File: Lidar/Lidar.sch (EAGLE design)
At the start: 4 parts

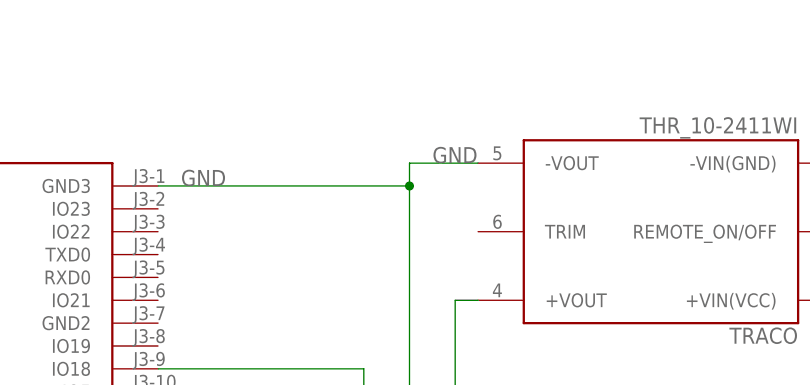
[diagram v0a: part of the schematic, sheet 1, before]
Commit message: board schematic
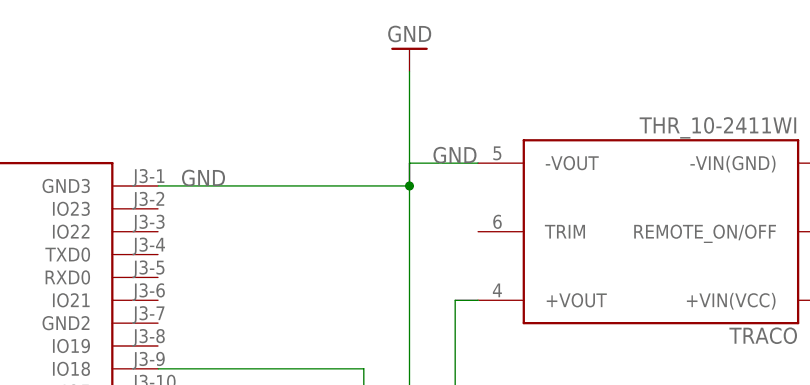
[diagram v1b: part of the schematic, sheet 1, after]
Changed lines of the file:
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@@
 <grid distance="0.1" unitdist="inch" unit="inch" style="lines" multiple="1" display="no" altdistance="0.01" altunitdist="inch" altunit="inch"/>
 <layers>
-<layer number="1" name="Top" color="4" fill="1" visible="yes" active="no"/>
-<layer number="16" name="Bottom" color="1" fill="1" visible="yes" active="no"/>
-<layer number="17" name="Pads" color="2" fill="1" visible="yes" active="no"/>
-<layer number="18" name="Vias" color="2" fill="1" visible="yes" active="no"/>
-<layer number="19" name="Unrouted" color="6" fill="1" visible="yes" active="no"/>
-<layer number="20" name="Dimension" color="15" fill="1" visible="yes" active="no"/>
-<layer number="21" name="tPlace" color="7" fill="1" visible="yes" active="no"/>
-<layer number="22" name="bPlace" color="7" fill="1" visible="yes" active="no"/>
-<layer number="23" name="tOrigins" color="15" fill="1" visible="yes" active="no"/>
-<layer number="24" name="bOrigins" color="15" fill="1" visible="yes" active="no"/>
-<layer number="25" name="tNames" color="7" fill="1" visible="yes" active="no"/>
-<layer number="26" name="bNames" color="7" fill="1" visible="yes" active="no"/>
-<layer number="27" name="tValues" color="7" fill="1" visible="yes" active="no"/>
-<layer number="28" name="bValues" color="7" fill="1" visible="yes" active="no"/>
+<layer number="1" name="Top" color="4" fill="1" visible="no" active="no"/>
+<layer number="16" name="Bottom" color="1" fill="1" visible="no" active="no"/>
+<layer number="17" name="Pads" color="2" fill="1" visible="no" active="no"/>
+<layer number="18" name="Vias" color="2" fill="1" visible="no" active="no"/>
+<layer number="19" name="Unrouted" color="6" fill="1" visible="no" active="no"/>
+<layer number="20" name="Dimension" color="15" fill="1" visible="no" active="no"/>
+<layer number="21" name="tPlace" color="7" fill="1" visible="no" active="no"/>
+<layer number="22" name="bPlace" color="7" fill="1" visible="no" active="no"/>
+<layer number="23" name="tOrigins" color="15" fill="1" visible="no" active="no"/>
+<layer number="24" name="bOrigins" color="15" fill="1" visible="no" active="no"/>
+<layer number="25" name="tNames" color="7" fill="1" visible="no" active="no"/>
+<layer number="26" name="bNames" color="7" fill="1" visible="no" active="no"/>
+<layer number="27" name="tValues" color="7" fill="1" visible="no" active="no"/>
+<layer number="28" name="bValues" color="7" fill="1" visible="no" active="no"/>
 <layer number="29" name="tStop" color="7" fill="3" visible="no" active="no"/>
 <layer number="30" name="bStop" color="7" fill="6" visible="no" active="no"/>
@@
 <layer number="35" name="tGlue" color="7" fill="4" visible="no" active="no"/>
 <layer number="36" name="bGlue" color="7" fill="5" visible="no" active="no"/>
-<layer number="37" name="tTest" color="7" fill="1" visible="yes" active="no"/>
-<layer number="38" name="bTest" color="7" fill="1" visible="yes" active="no"/>
+<layer number="37" name="tTest" color="7" fill="1" visible="no" active="no"/>
+<layer number="38" name="bTest" color="7" fill="1" visible="no" active="no"/>
 <layer number="39" name="tKeepout" color="4" fill="11" visible="no" active="no"/>
 <layer number="40" name="bKeepout" color="1" fill="11" visible="no" active="no"/>
@@
 <layer number="44" name="Drills" color="7" fill="1" visible="no" active="no"/>
 <layer number="45" name="Holes" color="7" fill="1" visible="no" active="no"/>
-<layer number="46" name="Milling" color="3" fill="1" visible="yes" active="no"/>
-<layer number="47" name="Measures" color="7" fill="1" visible="yes" active="no"/>
-<layer number="48" name="Document" color="7" fill="1" visible="yes" active="no"/>
-<layer number="49" name="Reference" color="7" fill="1" visible="yes" active="no"/>
-<layer number="50" name="dxf" color="7" fill="1" visible="yes" active="no"/>
-<layer number="51" name="tDocu" color="7" fill="1" visible="yes" active="no"/>
-<layer number="52" name="bDocu" color="7" fill="1" visible="yes" active="no"/>
-<layer number="53" name="tGND_GNDA" color="7" fill="9" visible="yes" active="no"/>
-<layer number="54" name="bGND_GNDA" color="1" fill="9" visible="yes" active="no"/>
-<layer number="56" name="wert" color="7" fill="1" visible="yes" active="no"/>
-<layer number="57" name="tCAD" color="7" fill="1" visible="yes" active="no"/>
-<layer number="58" name="bCAD" color="7" fill="1" visible="yes" active="no"/>
-<layer number="59" name="tCarbon" color="7" fill="1" visible="yes" active="no"/>
-<layer number="60" name="bCarbon" color="7" fill="1" visible="yes" active="no"/>
+<layer number="46" name="Milling" color="3" fill="1" visible="no" active="no"/>
+<layer number="47" name="Measures" color="7" fill="1" visible="no" active="no"/>
+<layer number="48" name="Document" color="7" fill="1" visible="no" active="no"/>
+<layer number="49" name="Reference" color="7" fill="1" visible="no" active="no"/>
+<layer number="50" name="dxf" color="7" fill="1" visible="no" active="no"/>
+<layer number="51" name="tDocu" color="7" fill="1" visible="no" active="no"/>
+<layer number="52" name="bDocu" color="7" fill="1" visible="no" active="no"/>
+<layer number="53" name="tGND_GNDA" color="7" fill="9" visible="no" active="no"/>
+<layer number="54" name="bGND_GNDA" color="1" fill="9" visible="no" active="no"/>
+<layer number="56" name="wert" color="7" fill="1" visible="no" active="no"/>
+<layer number="57" name="tCAD" color="7" fill="1" visible="no" active="no"/>
+<layer number="58" name="bCAD" color="7" fill="1" visible="no" active="no"/>
+<layer number="59" name="tCarbon" color="7" fill="1" visible="no" active="no"/>
+<layer number="60" name="bCarbon" color="7" fill="1" visible="no" active="no"/>
 <layer number="88" name="SimResults" color="9" fill="1" visible="yes" active="yes"/>
 <layer number="89" name="SimProbes" color="9" fill="1" visible="yes" active="yes"/>
@@
 </variantdefs>
 <classes>
-<class number="0" name="default" width="0" drill="0">
+<class number="0" name="default" width="0.8128" drill="0.1016">
+<clearance class="0" value="0.1016"/>
 </class>
 </classes>
@@
 <part name="CONN-LIDAR" library="SparkFun-Connectors" library_urn="urn:adsk.eagle:library:513" deviceset="CONN_05" device="PTH" package3d_urn="urn:adsk.eagle:package:38104/2"/>
 <part name="ESP32" library="ESP32-DEVKITC-32D" deviceset="ESP32-DEVKITC-32D" device=""/>
+<part name="GND1" library="supply1" library_urn="urn:adsk.eagle:library:371" deviceset="GND" device=""/>
 </parts>
 <sheets>
@@
 <attribute name="NAME" x="48.2428" y="104.8043" size="1.78" layer="95"/>
 <attribute name="VALUE" x="48.2437" y="50.7702" size="1.7799" layer="96"/>
+</instance>
+<instance part="GND1" gate="1" x="111.76" y="116.84" smashed="yes" rot="R180">
+<attribute name="VALUE" x="114.3" y="119.38" size="1.778" layer="96" rot="R180"/>
 </instance>
 </instances>
@@
 <label x="114.3" y="104.14" size="1.778" layer="95"/>
 <label x="86.36" y="101.6" size="1.778" layer="95"/>
-</segment>
-</net>
+<pinref part="GND1" gate="1" pin="GND"/>
+<wire x1="111.76" y1="101.6" x2="111.76" y2="114.3" width="0.1524" layer="91"/>
+</segment>
+</net>
